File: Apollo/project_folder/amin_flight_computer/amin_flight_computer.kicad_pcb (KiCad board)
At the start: 2 copper layers, 29 x 28 mm, 24 parts, among them J1 USB4105-GF-A-060, J3 Battery1, U1 LEA-M8T, U2 ESP32-S3-MINI-1, U3 XC6220B331MR, U4 TPD2EUSB30

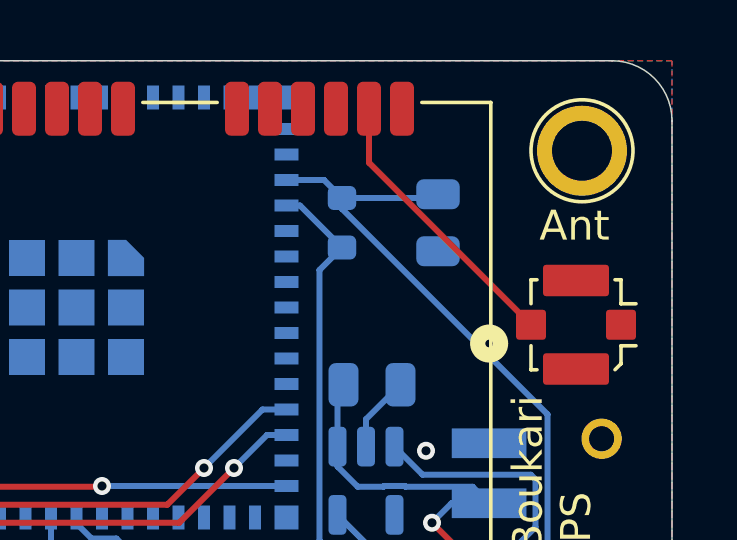
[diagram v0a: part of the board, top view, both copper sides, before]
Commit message: Amin has his 450th mg of caffeine and realizes thicc traces more better
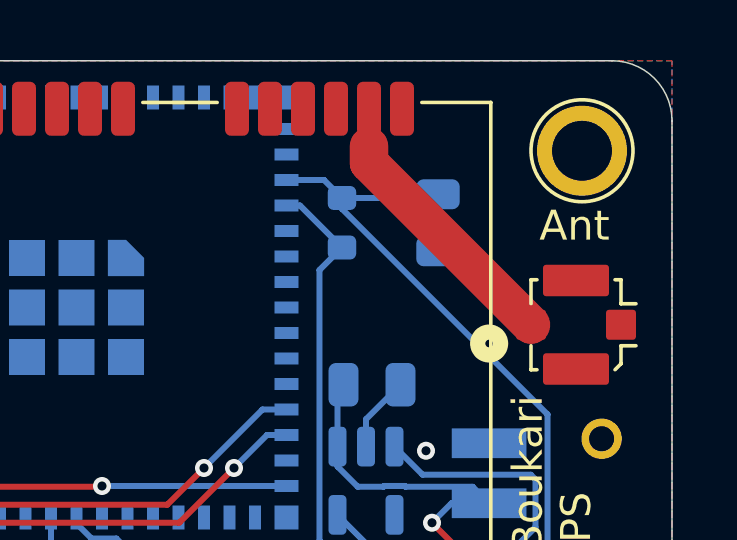
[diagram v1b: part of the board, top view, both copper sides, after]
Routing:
- net Net-(J2-In): track 9.44 -> 8.19 mm
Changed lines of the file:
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@@
 	(segment
 		(start 151.9 66.4)
-		(end 151.9 64.6)
-		(width 0.2)
+		(end 151.9 65.85)
+		(width 1.2842)
 		(layer "F.Cu")
 		(net 4)
@@
 		(start 157.3 71.8)
 		(end 151.9 66.4)
-		(width 0.2)
+		(width 1.2842)
 		(layer "F.Cu")
 		(net 4)
